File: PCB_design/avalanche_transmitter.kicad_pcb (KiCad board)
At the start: 2 copper layers, 22 parts, among them J1 Conn_01x07_Pin, Q1 2N3904, U1 74HC00

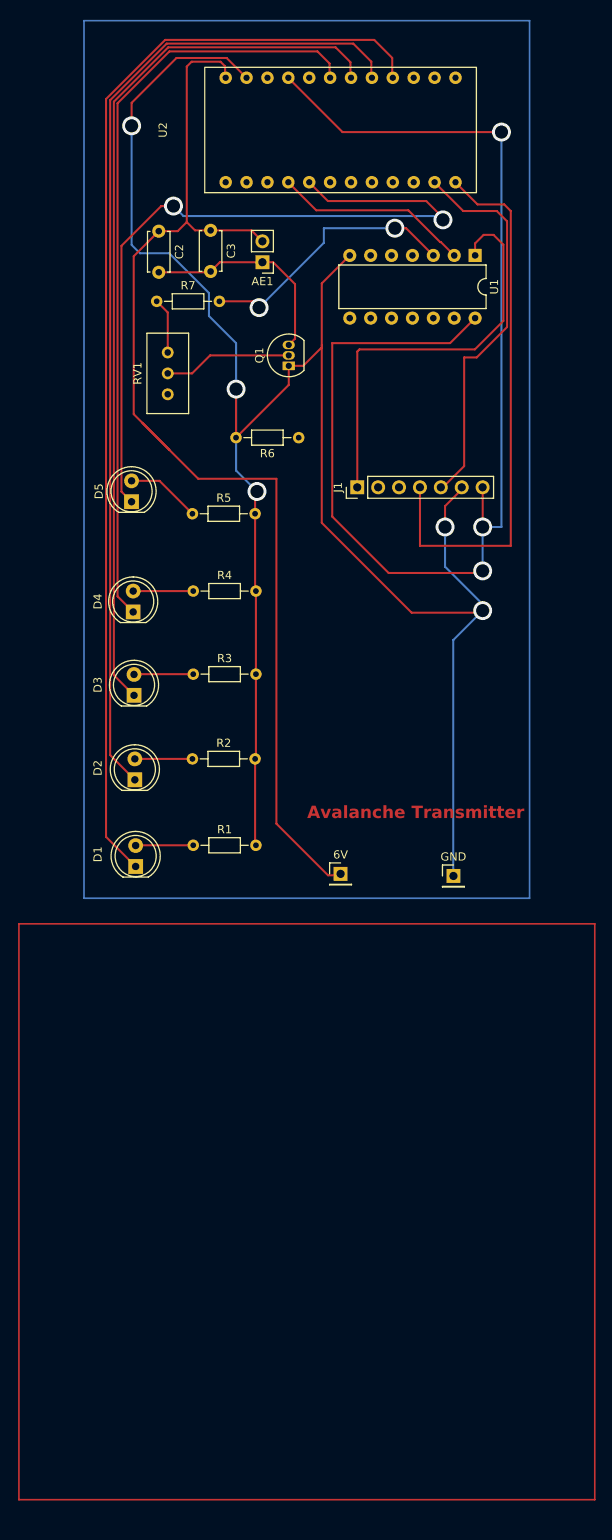
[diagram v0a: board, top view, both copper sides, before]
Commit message: finished PCB. ready for bens review
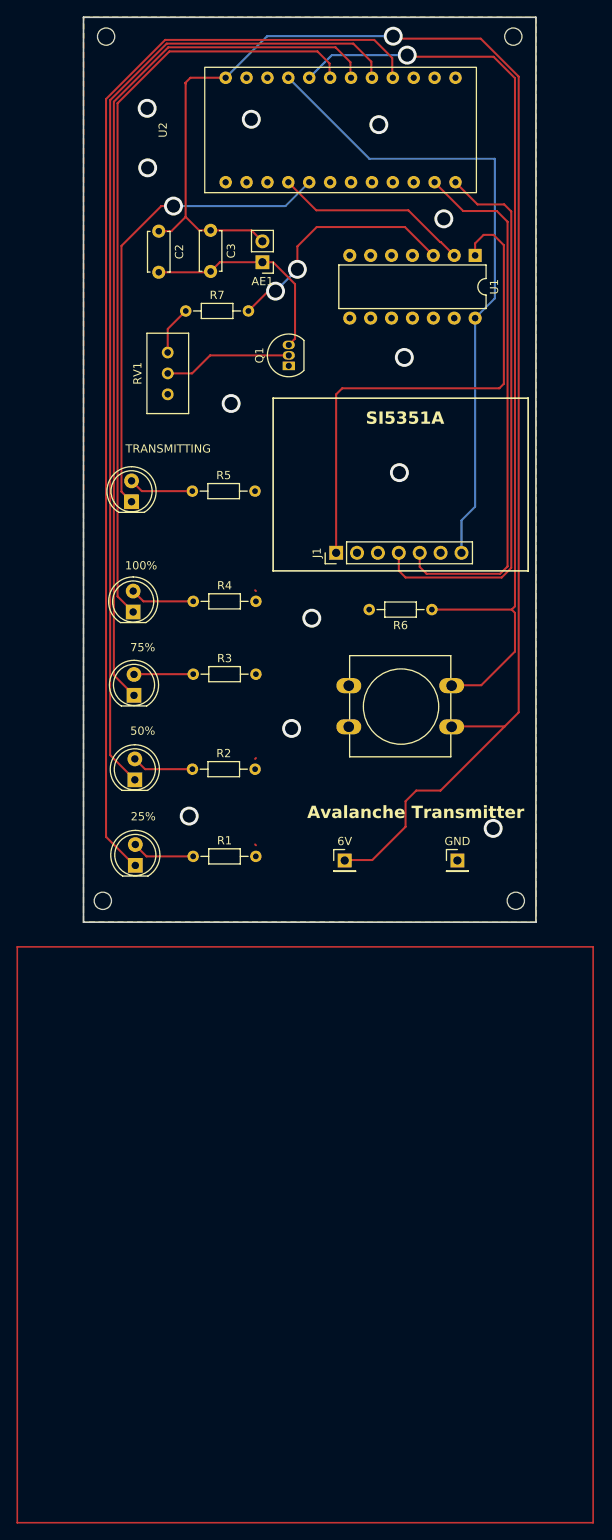
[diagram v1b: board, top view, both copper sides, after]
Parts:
- removed D1: RED_LED_25, LED_THT:LED_D5.0mm
- added 25%: RED_LED_25, LED_THT:LED_D5.0mm, F.Cu at (38.5, 118.1)
- added REF**: MountingHole_2.1mm, MountingHole:MountingHole_2.1mm, F.Cu at (34.6, 122.4)
- added REF**: MountingHole_2.1mm, MountingHole:MountingHole_2.1mm, F.Cu at (84.5, 17.4)
- added REF**: MountingHole_2.1mm, MountingHole:MountingHole_2.1mm, F.Cu at (35.0, 17.4)
- added REF**: MountingHole_2.1mm, MountingHole:MountingHole_2.1mm, F.Cu at (84.8, 122.4)
- added REF**: SW_PUSH-12mm, Button_Switch_THT:SW_PUSH-12mm, F.Cu at (64.5, 96.2)
- moved R6 26.4 mm to (74.6, 87.0)
- moved J1 8.37 mm to (63.0, 80.1)
- moved R7 3.72 mm to (44.7, 50.7)
- moved R5 2.75 mm to (45.5, 72.6)
- moved GND 1.94 mm to (77.7, 117.5)
- moved 6V 1.70 mm to (64.0, 117.5)
- moved R1 1.35 mm to (45.6, 117.0)
- moved R2 1.25 mm to (45.5, 106.4)
- moved R4 1.25 mm to (45.6, 86.0)
- renumbered D4 to 100%, D2 to 50%, D3 to 75%, D5 to TRANSMITTING
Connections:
- 100% pad 1: Net-(D4-K) -> Net-(D1-K)
- 50% pad 1: Net-(D2-K) -> Net-(D3-K)
- 6V pad 1: (no net) -> +6V
- 75% pad 1: Net-(D3-K) -> Net-(D2-K)
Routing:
- net GND: track 248.0 -> 0.42 mm, vias 5 -> 12
- net Net-(U2-8): track 0.00 -> 116.6 mm, vias 0 -> 1
- net +3V0: track 149.9 -> 78.8 mm, vias 3 -> 0
- net +6V: track 140.0 -> 190.0 mm, vias 0 -> 1
- net Net-(D4-K): track 93.3 -> 135.8 mm
- net Net-(D1-K): track 135.8 -> 93.3 mm
- net Net-(D5-K): track 91.6 -> 57.4 mm, vias 2 -> 1
- net Net-(J1-Pin_5): track 47.7 -> 66.0 mm
- net Net-(D3-K): track 107.3 -> 121.3 mm
- net Net-(D2-K): track 121.3 -> 107.3 mm
- net Net-(J1-Pin_1): track 51.1 -> 62.9 mm
- net Net-(R7-Pad2): track 32.7 -> 29.8 mm
- net Net-(J1-Pin_4): track 66.9 -> 68.3 mm
- net Net-(D5-A): track 9.06 -> 7.91 mm
- net Net-(R7-Pad1): track 6.92 -> 5.96 mm
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- added copper zone on B.Cu, net GND
- added copper zone on F.Cu, net GND
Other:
- board outline added: 55 x 110 mm
- board text added: "SI5351A"
